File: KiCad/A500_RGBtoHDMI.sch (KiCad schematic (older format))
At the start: 5 parts, among them J1 Conn_02x20_Odd_Even, J2 Conn_01x06, U1 Denise_Socket, U2 XC9572XL-VQ64, U3 Denise_MB_PinHeader

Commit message: more routing and fixes
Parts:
- J1: symbol Connector_Generic:Conn_02x20_Odd_Even -> A500_RGBtoHDMI:RPi_Zero_Conn_02x20_Odd_Even
- renumbered J2 to JTAG1
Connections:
- net CBL is gone; now on net CSYNC: U1.32 (BLANK), U3.32 (BLANK)
- net GPIO10 is gone; now on net R0_3V3: J1.19 (GPIO10)
- net GPIO11 is gone; now on net R1_3V3: J1.23 (GPIO11)
- net GPIO12 is gone; now on net R2_3V3: J1.32 (GPIO12)
- net GPIO13 is gone; now on net R3_3V3: J1.33 (GPIO13)
- net GPIO17 is gone; now on net PSYNC: J1.11 (GPIO17)
- net GPIO18 is gone; now on net VERSION: J1.12 (GPIO18)
- net GPIO2 is gone; now on net B0_3V3: J1.3 (GPIO2)
- net GPIO20 is gone; now on net SPCLK: J1.38 (GPIO20)
- net GPIO21 is gone; now on net CLK: J1.40 (GPIO21)
- net GPIO23 is gone; now on net CSYNC_3V3: J1.16 (GPIO23)
- net GPIO3 is gone; now on net B1_3V3: J1.5 (GPIO3)
- net GPIO4 is gone; now on net B2_3V3: J1.7 (GPIO4)
- net GPIO5 is gone; now on net B3_3V3: J1.29 (GPIO5)
- net GPIO6 is gone; now on net G0_3V3: J1.31 (GPIO6)
- net GPIO7 is gone; now on net G1_3V3: J1.26 (GPIO7)
- net GPIO8 is gone; now on net G2_3V3: J1.24 (GPIO8)
- net GPIO9 is gone; now on net G3_3V3: J1.21 (GPIO9)
- net B0: now also U2.56 (FB4-15)
- net B1: now also U2.57 (FB4-17)
- net B2: now also U2.58 (FB2-3)
- net B3: now also U2.59 (FB2-4)
- net G0: now also U2.60 (FB2-2)
- net G1: now also U2.61 (FB2-5)
- net G2: now also U2.62 (FB2-6)
- net G3: now also U2.63 (FB2-8)
- net R0: now also U2.49 (FB4-6)
- net R1: now also U2.50 (FB4-14)
- net R2: now also U2.51 (FB4-10)
- net R3: now also U2.52 (FB4-12)
- net B0_3V3: now reaches U2.1 (FB2-10)
- net B3_3V3: now reaches U2.10 (FB1-6)
- net G0_3V3: now reaches U2.11 (FB1-8)
- net G2_3V3: now reaches U2.12 (FB1-3)
- net G1_3V3: now reaches U2.13 (FB1-4)
- net CLK: now reaches U2.15 (FB1-9/GCK1)
- net SPCLK: now reaches U2.16 (FB1-11/GCK2)
- net CSYNC: now reaches U2.17 (FB1-14/GCK3)
- net R2_3V3: now reaches U2.18 (FB1-10)
- net R3_3V3: now reaches U2.19 (FB1-15)
- net B1_3V3: now reaches U2.2 (FB2-11/GTS2)
- net B2_3V3: now reaches U2.4 (FB2-12)
- net PSYNC: now reaches U2.5 (FB2-14/GTS1)
- net CSYNC_3V3: now reaches U2.6 (FB2-15)
- net VERSION: now reaches U2.64 (FB2-9/GSR)
- net R0_3V3: now reaches U2.7 (FB2-17)
- net G3_3V3: now reaches U2.8 (FB1-2)
- net R1_3V3: now reaches U2.9 (FB1-5)
- net GPIO0: no longer names the net of J1.27 (GPIO0)
- net GPIO1: no longer names the net of J1.28 (GPIO1)
- net GPIO14: no longer names the net of J1.8 (GPIO14)
- net GPIO15: no longer names the net of J1.10 (GPIO15)
- net GPIO16: no longer names the net of J1.36 (GPIO16)
- net GPIO19: no longer names the net of J1.35 (GPIO19)
- net GPIO22: no longer names the net of J1.15 (GPIO22)
- net GPIO24: no longer names the net of J1.18 (GPIO24)
- net GPIO25: no longer names the net of J1.22 (GPIO25)
- net GPIO26: no longer names the net of J1.37 (GPIO26)
- net GPIO27: no longer names the net of J1.13 (GPIO27)
- net ZD renamed PIXELSW
- no-connect marks 2 -> 13
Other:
- moved on the sheet: J1

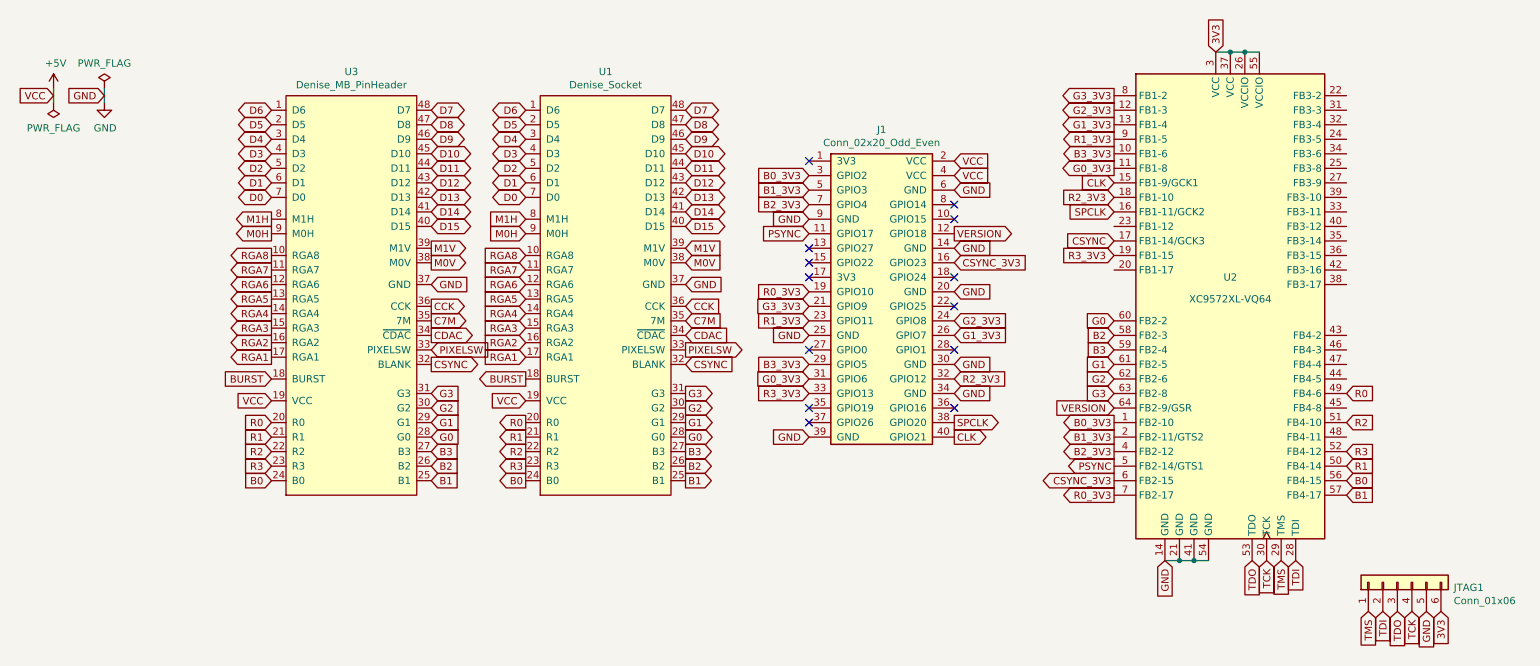
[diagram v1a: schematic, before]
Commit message: more routing and small adjustments,fixes and improvements
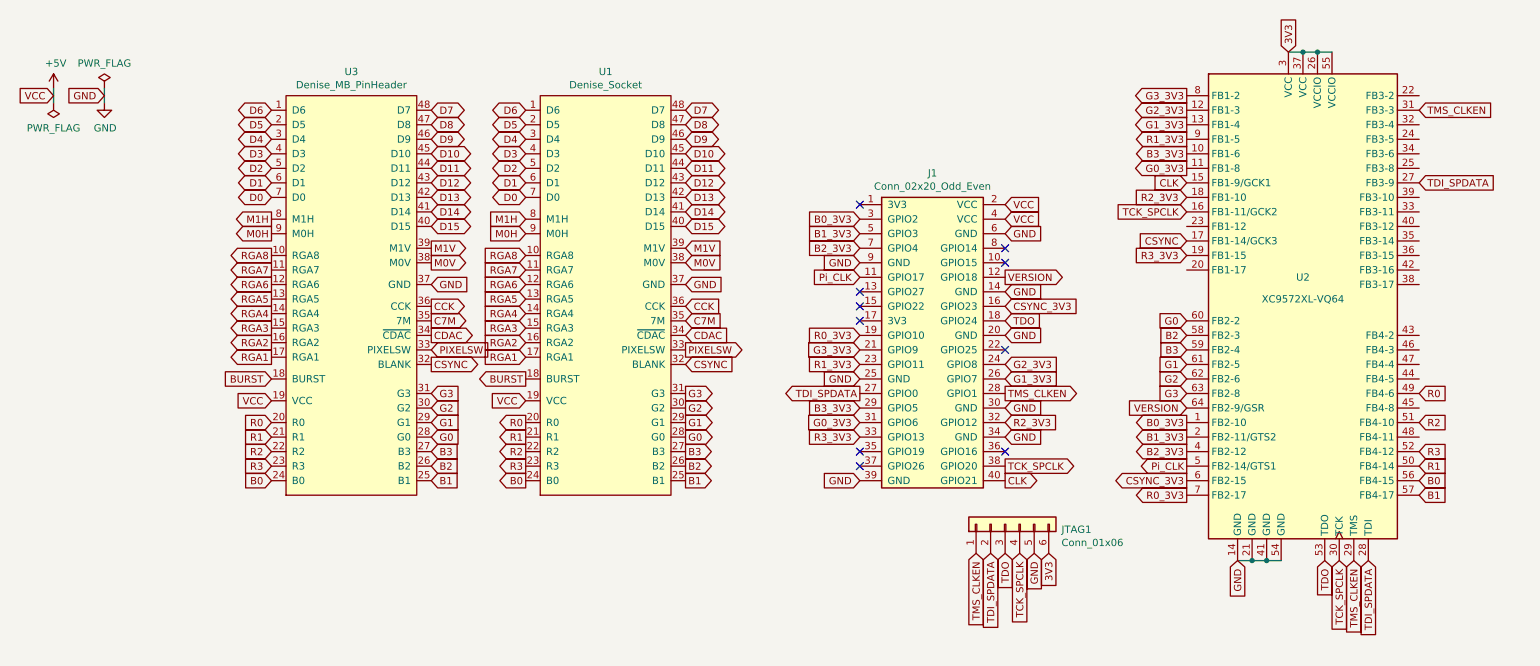
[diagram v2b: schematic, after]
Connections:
- net TCK is gone; now on net TCK_SPCLK: JTAG1.4 (Pin_4), U2.30 (TCK)
- net TDI is gone; now on net TDI_SPDATA: JTAG1.2 (Pin_2), U2.28 (TDI)
- net TMS is gone; now on net TMS_CLKEN: JTAG1.1 (Pin_1), U2.29 (TMS)
- net TDO: now also J1.18 (GPIO24)
- net TDI_SPDATA: now reaches J1.27 (GPIO0)
- net TDI_SPDATA: now also U2.27 (FB3-9)
- net TMS_CLKEN: now reaches J1.28 (GPIO1)
- net TMS_CLKEN: now also U2.31 (FB3-3)
- net PSYNC renamed Pi_CLK
- net SPCLK renamed TCK_SPCLK
- no-connect marks 13 -> 10
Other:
- moved on the sheet: J1, JTAG1, U2
